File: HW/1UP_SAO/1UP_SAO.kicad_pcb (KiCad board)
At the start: 2 copper layers, 48 x 48 mm, 17 parts, among them X1 Badgelife_sao_connector_v169b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

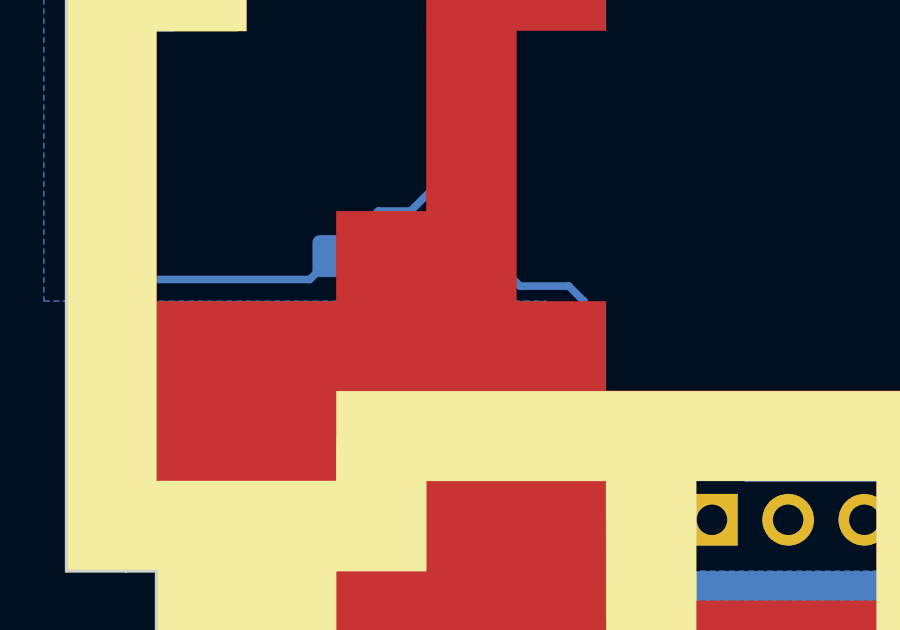
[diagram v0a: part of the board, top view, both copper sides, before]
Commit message: done?
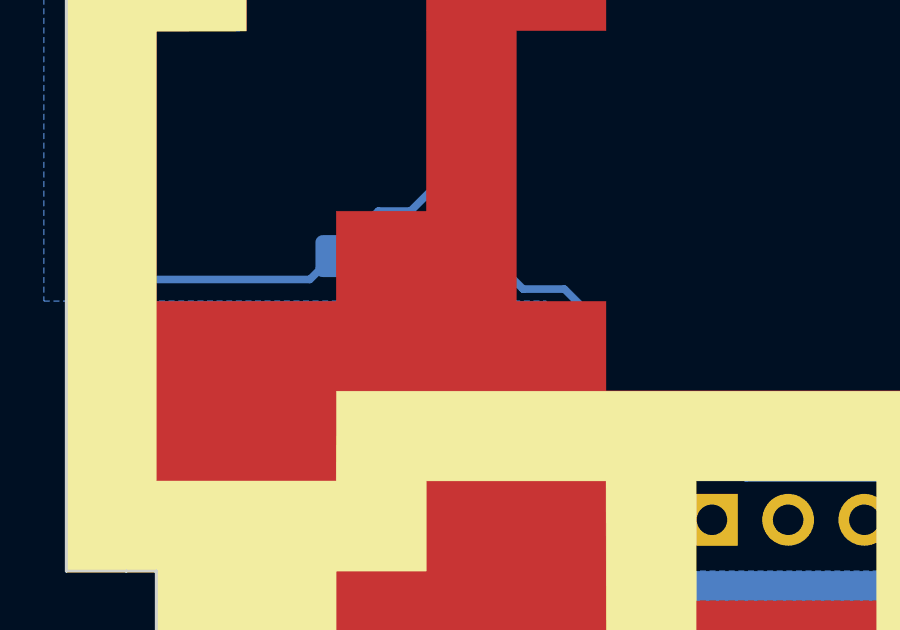
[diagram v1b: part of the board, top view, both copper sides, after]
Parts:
- moved R1 0.10 mm to (85.9, 101.5)
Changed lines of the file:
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@@
   )
   (module Resistor_SMD:R_0805_2012Metric_Pad1.15x1.40mm_HandSolder (layer B.Cu)
-    (at 85.8 101.5 180)
+    (at 85.9 101.5 180)
     (descr "Resistor SMD 0805 (2012 Metric), square (rectangular) end terminal, IPC_7351 nominal with elongated pad for handsoldering. (Body size source: https://docs.google.com/spreadsheets/d/1BsfQQcO9C6DZCsRaXUlFlo91Tg2WpOkGARC1WS5S8t0/edit?usp=sharing), generated with kicad-footprint-generator")
     (tags "resistor handsolder")
@@
   (segment (start 111.19559 102.27941) (end 111.975 101.5) (width 0.254) (layer B.Cu) (net 8))
   (segment (start 107.47059 102.27941) (end 111.19559 102.27941) (width 0.254) (layer B.Cu) (net 8))
-  (segment (start 92.75 102.5) (end 91.125 102.5) (width 0.254) (layer B.Cu) (net 8))
-  (segment (start 93.25 103) (end 92.75 102.5) (width 0.254) (layer B.Cu) (net 8))
+  (segment (start 111.975 101.5) (end 113.075 101.5) (width 0.254) (layer B.Cu) (net 8))
+  (segment (start 92.6 102.6) (end 91.225 102.6) (width 0.254) (layer B.Cu) (net 8))
+  (segment (start 93.25 103.25) (end 92.6 102.6) (width 0.254) (layer B.Cu) (net 8))
   (segment (start 97.52 107.75) (end 96.656401 106.886401) (width 0.254) (layer B.Cu) (net 8))
+  (segment (start 90.225 101.6) (end 87.2 101.6) (width 0.254) (layer B.Cu) (net 8))
   (segment (start 96.656401 106.886401) (end 94.136401 106.886401) (width 0.254) (layer B.Cu) (net 8))
-  (segment (start 91.125 102.5) (end 90.225 101.6) (width 0.254) (layer B.Cu) (net 8))
+  (segment (start 91.225 102.6) (end 90.225 101.6) (width 0.254) (layer B.Cu) (net 8))
   (segment (start 94.136401 106.886401) (end 93.25 106) (width 0.254) (layer B.Cu) (net 8))
-  (segment (start 90.225 101.6) (end 87.2 101.6) (width 0.254) (layer B.Cu) (net 8))
-  (segment (start 93.25 106) (end 93.25 103) (width 0.254) (layer B.Cu) (net 8))
-  (segment (start 111.975 101.5) (end 113.075 101.5) (width 0.254) (layer B.Cu) (net 8))
+  (segment (start 93.25 106) (end 93.25 103.25) (width 0.254) (layer B.Cu) (net 8))
   (zone (net 2) (net_name GND) (layer B.Cu) (hatch edge 0.508)
     (connect_pads (clearance 0))
